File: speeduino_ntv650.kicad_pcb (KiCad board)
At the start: 2 copper layers, 105.1 x 96.7 mm, 70 parts, among them IC1 SP721, IC2 TC4424, J1 Conn_01x25_DB-25, P1 MAX9926_9927, Q1 STP62NS04Z, Q2 STP62NS04Z, Q3 STP62NS04Z, U1 LM2937xT

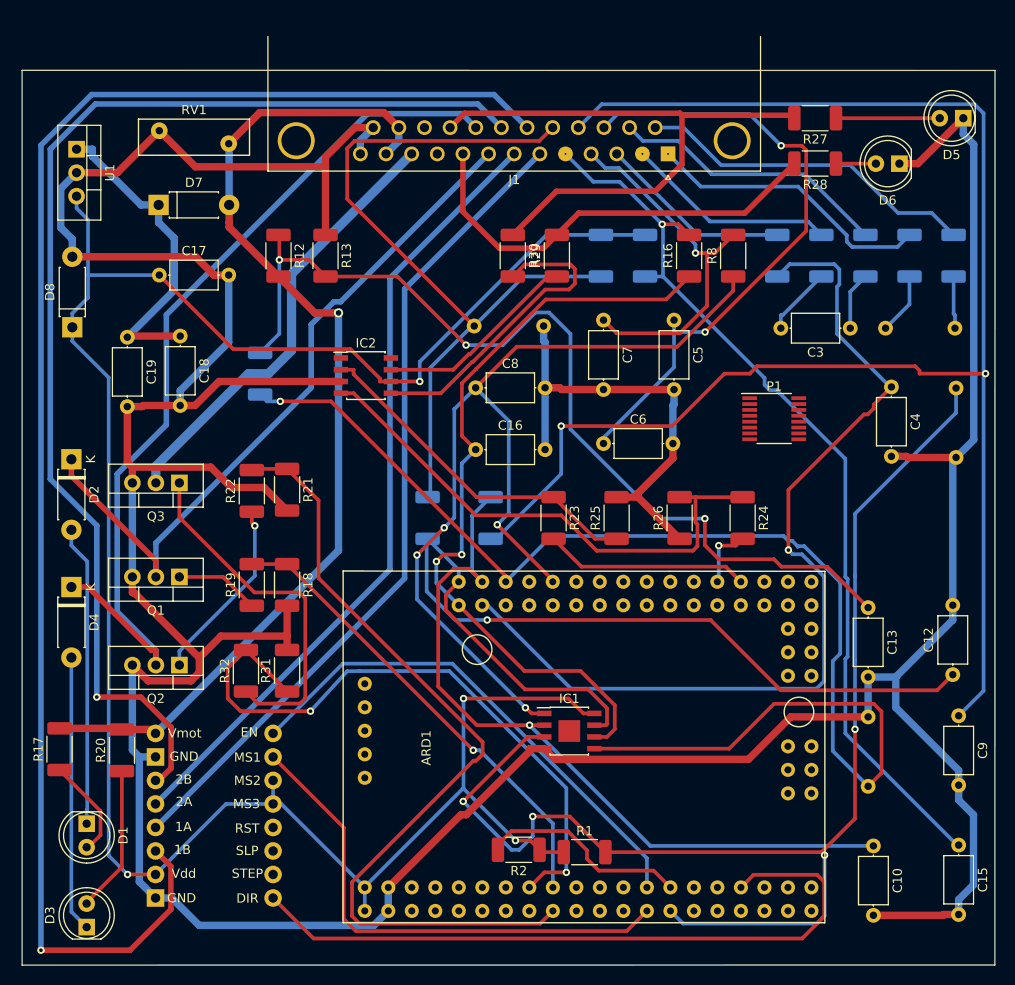
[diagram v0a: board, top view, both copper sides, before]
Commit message: first complited pcb
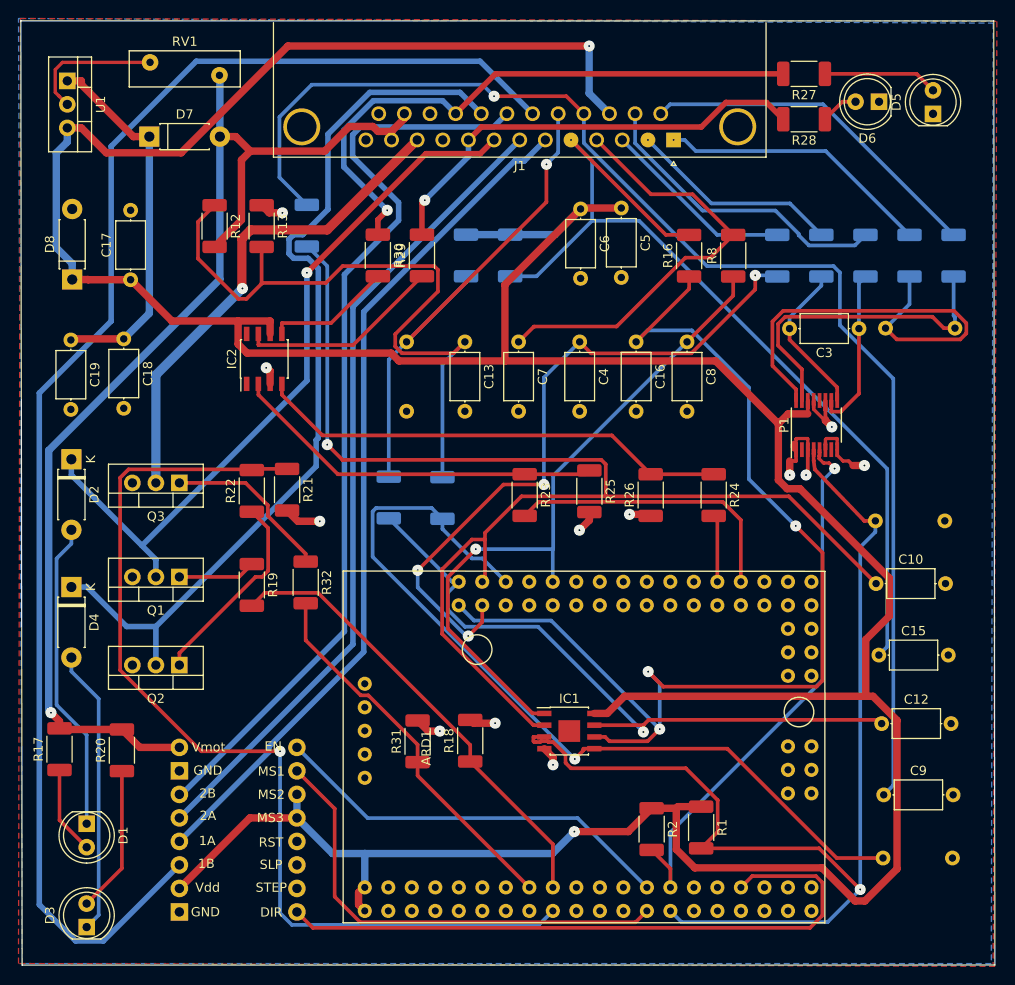
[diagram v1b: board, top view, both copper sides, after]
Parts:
- moved C13 52.2 mm to (108.2, 55.2)
- moved R9 37.3 mm to (91.2, 42.7), turned to 90 degrees
- moved C4 34.0 mm to (120.6, 55.2)
- moved C10 28.3 mm to (152.7, 81.3), turned to 0 degrees
- moved R18 26.0 mm to (108.8, 98.3), turned to 90 degrees
- moved C6 25.5 mm to (120.7, 40.9), turned to 270 degrees
- moved R14 23.8 mm to (105.8, 72.1)
- moved C8 23.4 mm to (132.2, 55.2), turned to 270 degrees
- moved C15 22.3 mm to (152.9, 89.1), turned to 0 degrees
- moved C16 20.9 mm to (126.7, 55.2), turned to 270 degrees
- moved R31 16.0 mm to (103.1, 98.4)
- moved R10 14.6 mm to (108.3, 45.9)
- moved R15 14.6 mm to (113.1, 45.9)
- moved R29 14.6 mm to (103.6, 45.9)
- moved R30 14.6 mm to (98.8, 45.9)
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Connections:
- C5 pad 1: MAP_5V -> 5V
- C6 pad 1: MAP_5V -> 5V
- J1 pad 16: MAP_5V -> 5V
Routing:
- net GND: track 485.5 -> 62.9 mm, vias 0 -> 12
- net 5V: track 240.8 -> 412.2 mm, vias 4 -> 2
- net MAP_5V: track 68.1 -> 0.00 mm, vias 2 -> 0
- net ADC-Clamp3: track 83.5 -> 138.1 mm
- net ADC-Clamp4: track 141.6 -> 93.0 mm
- net Net-(C2-Pad1): track 6.65 -> 49.4 mm
- net TACH2-CPU-D18: track 22.9 -> 60.9 mm, vias 0 -> 1
- net ADC-Clamp2: track 84.3 -> 121.2 mm, vias 2 -> 3
- net TPS_sens: track 176.4 -> 142.2 mm, vias 2 -> 1
- net Net-(C2-Pad2): track 5.64 -> 36.6 mm
- net ADC-Clamp1: track 103.5 -> 73.4 mm, vias 4 -> 1
- net ADC-Clamp6: track 102.3 -> 72.7 mm
- net Net-(C13-Pad1): track 103.4 -> 73.9 mm, vias 3 -> 0
- net IDLE-CPU-D6: track 70.5 -> 41.2 mm, vias 2 -> 0
- net MAP-CPU-A3: track 102.6 -> 74.2 mm, vias 1 -> 4
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- added copper zone on F.Cu, net (none)
- added copper zone on B.Cu, net GND
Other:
- board size 105.1 x 96.7 mm -> 105.2 x 102 mm
- net class 5v_small: clearance 0.11 -> 0.2; via_dia 0.8 -> 1.2; via_drill 0.4 -> 0.2
- net class Default: clearance 0.4 -> 0.2; via_dia 0.8 -> 1.2; via_drill 0.4 -> 0.2
- net class GND_MOSFIT: clearance 0.4 -> 0.3; via_dia 1 -> 1.2; via_drill 0.8 -> 0.2
- net class POWER_ENG: clearance 0.4 -> 0.28; via_dia 0.8 -> 1.2; via_drill 0.4 -> 0.2
- net class Power: clearance 0.4 -> 0.22; via_dia 1 -> 1.2; via_drill 0.6 -> 0.2
- net class power_exit: clearance 0.4 -> 0.3; via_dia 0.8 -> 1.2; via_drill 0.4 -> 0.2
- net class power_logic: via_dia 0.8 -> 1.2; via_drill 0.7 -> 0.2
- net class step_engine_exit: clearance 0.4 -> 0.3; via_dia 0.8 -> 1.2; via_drill 0.4 -> 0.2
- rule trace_clearance: 0.4 -> 0.2
- rule via_min_drill: 0.3 -> 0.2
- rule via_min_size: 0.4 -> 0.1
